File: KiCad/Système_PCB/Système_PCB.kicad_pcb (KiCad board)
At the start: 2 copper layers, 8 parts, among them J1 Autocom4, J2 Omnimate2, J3 Omnimate2, Q1 IRL510

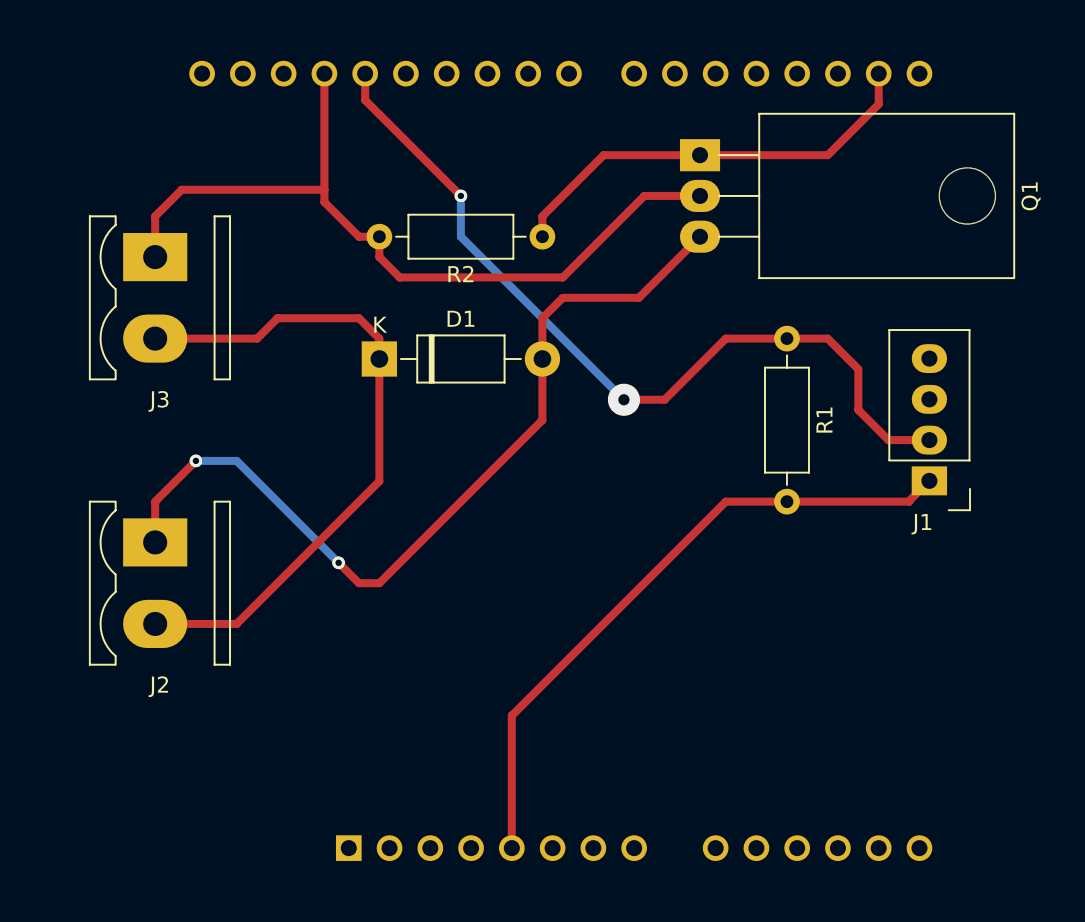
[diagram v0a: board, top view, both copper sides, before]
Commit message: Change PCB
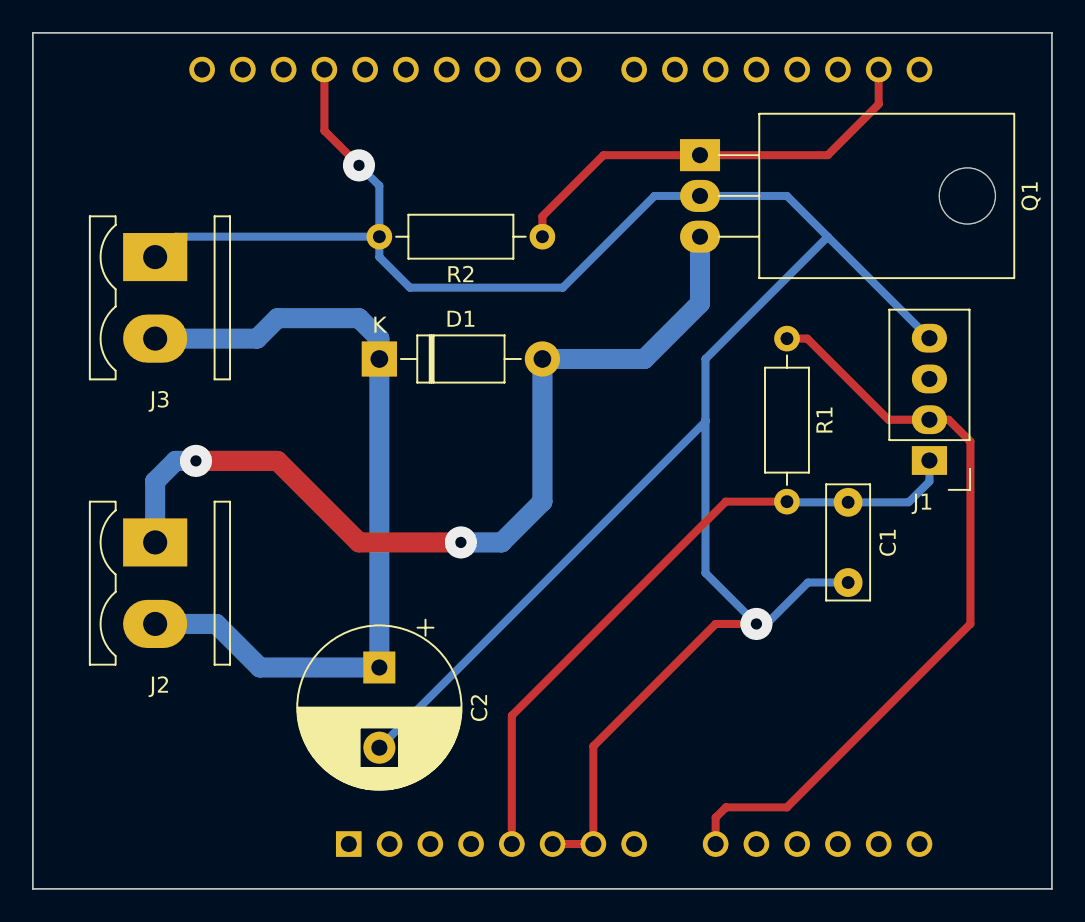
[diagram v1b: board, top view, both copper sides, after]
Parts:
- added C1: C, FootprintGamelGe2_v6:C_Rect_L7.0mm_W2.5mm_P5.00mm, F.Cu at (246.4, 81.3)
- added C2: Cp, FootprintGamelGe2_v6:CP_Radial_D10.0mm_P5.00mm, F.Cu at (217.2, 91.6)
- moved J1 1.27 mm to (251.4, 78.7)
- moved A1 0.25 mm to (215.3, 102.6)
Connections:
- A1 pad 28: /D13 -> unconnected-(A1-Pad28)
- A1 pad 6: unconnected-(A1-Pad6) -> GND
- A1 pad 7: unconnected-(A1-Pad7) -> GND
- A1 pad 9: unconnected-(A1-Pad9) -> /A0
- J1 pad 2: /D13 -> /A0
- R1 pad 1: /D13 -> /A0
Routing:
- net GND: track 50.0 -> 154.9 mm, vias 0 -> 2
- net /D13: track 54.3 -> 0.00 mm, vias 2 -> 0
- net /A0: track 0.00 -> 48.0 mm
- net +12V: track 41.6 -> 50.6 mm
- net /5V: track 44.8 -> 41.4 mm
- net Net-(D1-Pad2): track 53.4 -> 55.9 mm
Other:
- board outline added: 63.5 x 53.3 mm
